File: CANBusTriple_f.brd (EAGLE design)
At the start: 50.2 x 49.5 mm, 63 parts, among them IC4 MCP1703CB, IC6 IC_MEM_23LC1024, U1 BLE112

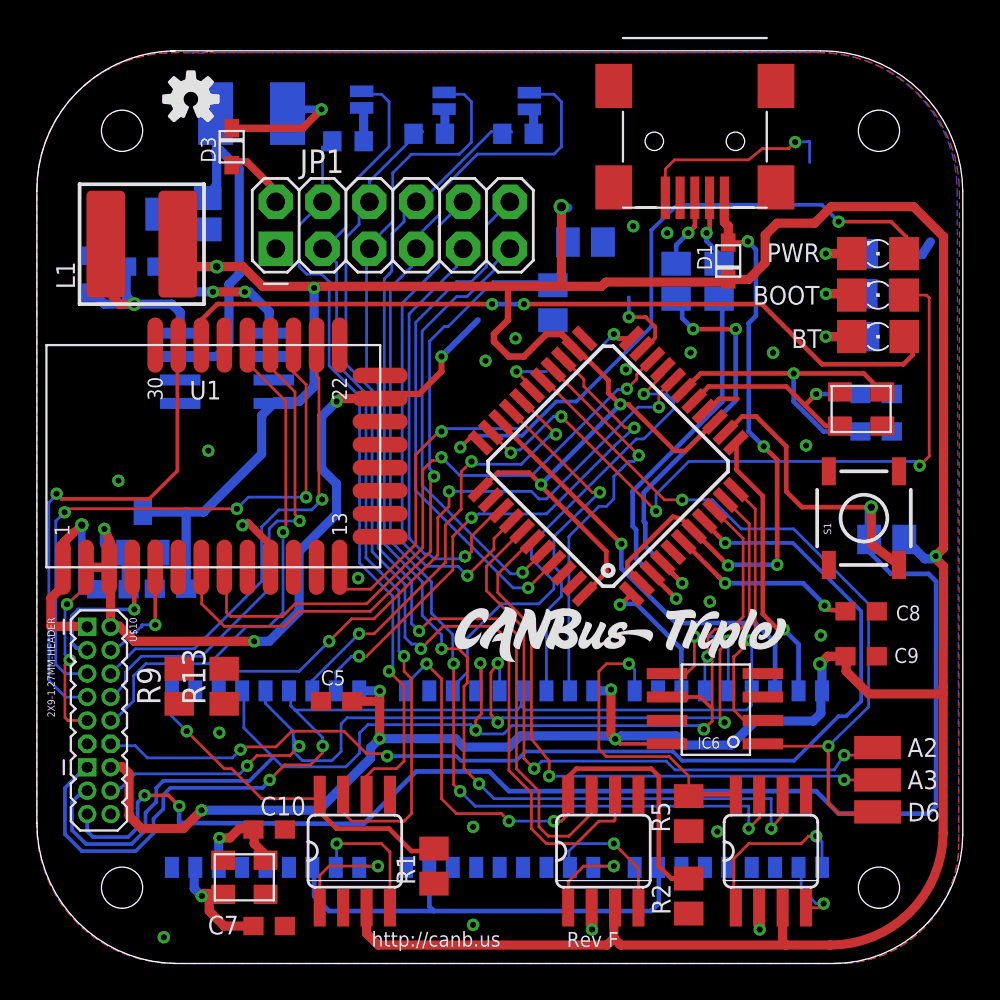
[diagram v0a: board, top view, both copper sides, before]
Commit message: Last sleep mode tweak, added line from BT LE to CAN1INT to wake the MCU up via BT
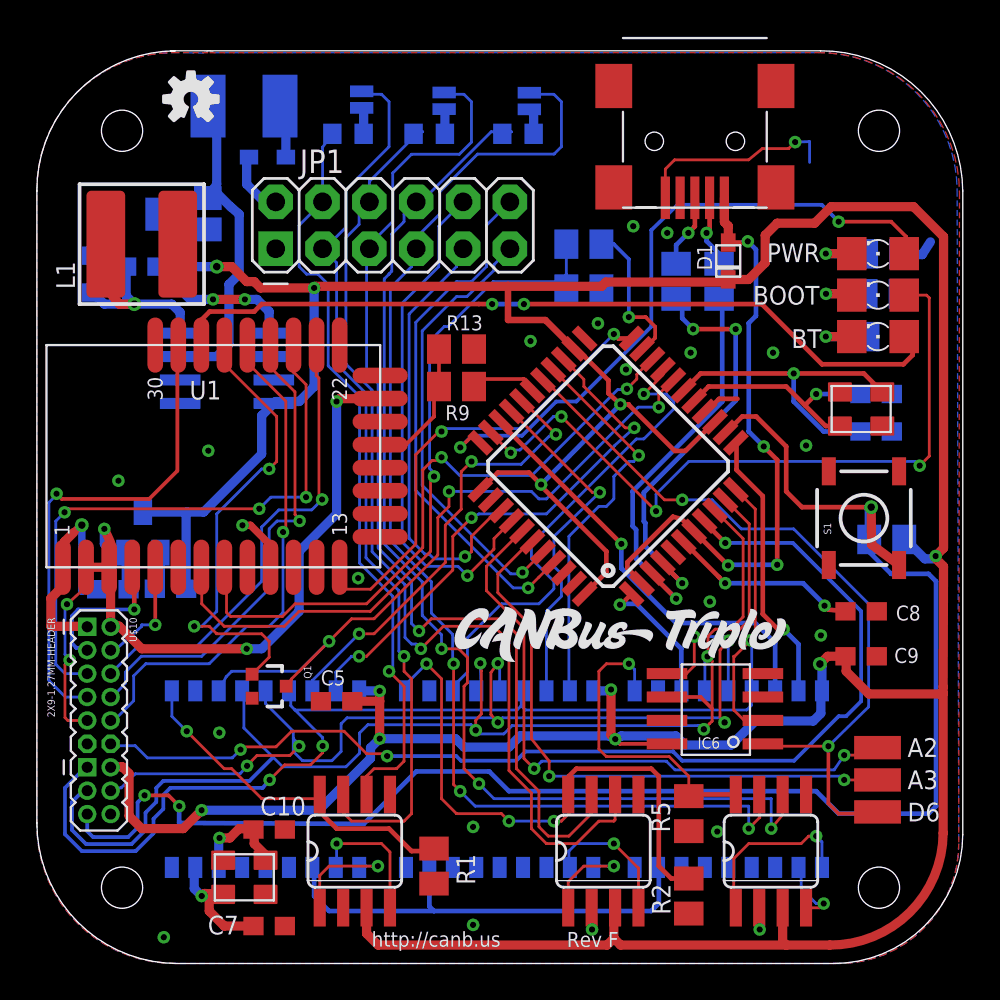
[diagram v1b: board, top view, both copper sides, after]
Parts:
- added Q1: MOSFET-NCHANNEL2N7002PW, SparkFun-DiscreteSemi:SOT323
- L1: value 47uH -> 68uH
- moved R13 22.2 mm to (22.8, 33.3), turned to 180 degrees
- moved R9 22.1 mm to (22.8, 31.3), turned to 0 degrees
- moved D3 2.02 mm to (12.5, 43.7), flipped to the bottom, turned to 180 degrees
- moved R10 1.83 mm to (29.7, 36.6), turned to 0 degrees
- moved F1 0.57 mm to (11.2, 46.5)
- moved CAN1-TRM 0.41 mm to (16.9, 45.0)
- moved R11 0.14 mm to (29.7, 39.0), turned to 180 degrees
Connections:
- new net N$33: Q1.1, U1.P0_1
- net +5V: no longer L1.2
- net CAN1_INT: now also Q1.3
- net GND: now also Q1.2
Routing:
- net N$33: track 0.00 -> 25.3 mm, vias 0 -> 2
- net +5V: track 259.0 -> 248.7 mm, vias 12 -> 11
- net +3V: track 58.8 -> 50.8 mm, vias 6 -> 5
- net N$29: track 0.00 -> 7.65 mm
- net N$22: track 7.25 -> 2.90 mm, vias 1 -> 0
- net N$19: track 4.28 -> 8.17 mm
- net CAN1_INT: track 34.2 -> 37.6 mm
- net N$38: track 36.0 -> 39.3 mm
- net GND: track 34.9 -> 36.9 mm
- net SUPPLY: track 19.1 -> 18.1 mm
- net N$36: track 3.21 -> 3.89 mm, vias 1 -> 0

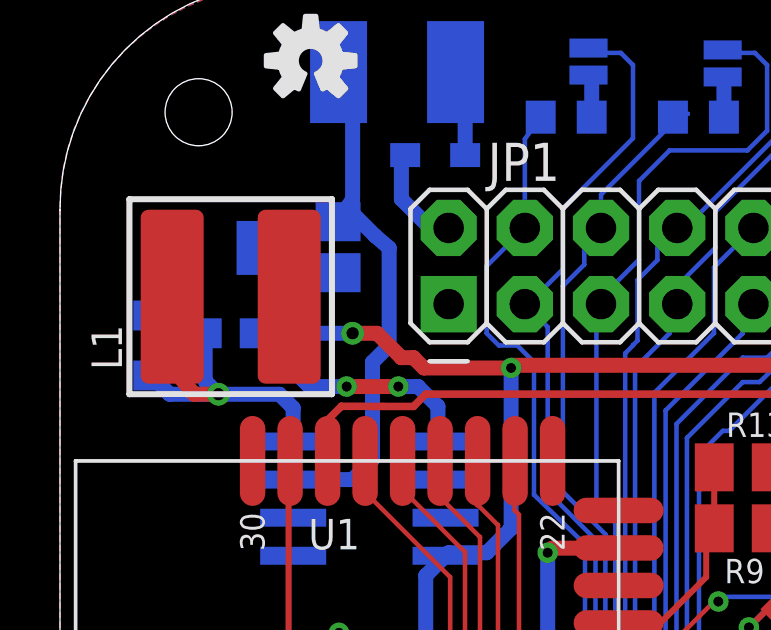
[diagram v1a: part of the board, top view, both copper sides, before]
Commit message: Fix missing trace on inductor
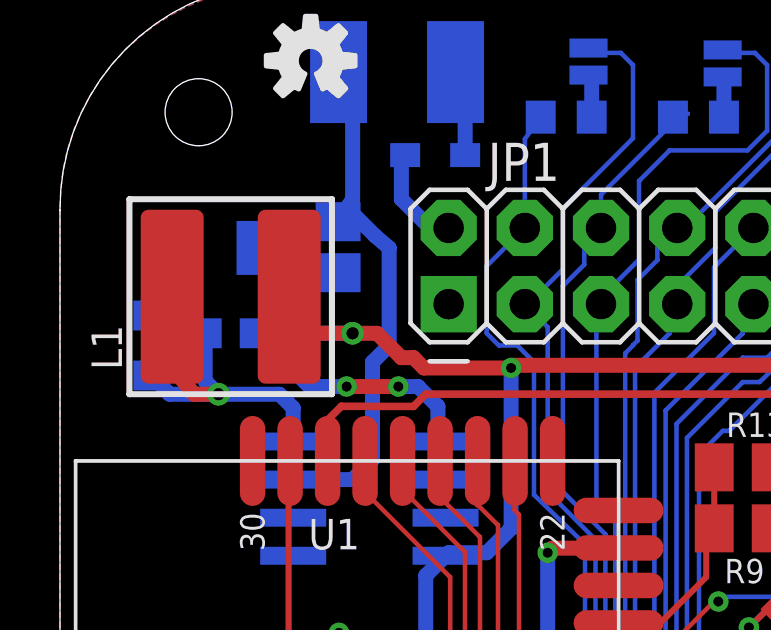
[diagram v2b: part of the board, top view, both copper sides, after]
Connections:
- net +5V: now also L1.2
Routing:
- net +5V: track 248.7 -> 251.5 mm
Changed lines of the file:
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@@
 <wire x1="11.3792" y1="36.9824" x2="10.5664" y2="37.7952" width="0.5" layer="1"/>
 <wire x1="10.5664" y1="37.7952" x2="9.7536" y2="37.7952" width="0.5" layer="1"/>
+<contactref element="L1" pad="2"/>
+<wire x1="7.6396" y1="39.0144" x2="7.6396" y2="38.69" width="0.5" layer="1"/>
+<wire x1="7.6396" y1="38.69" x2="8.5344" y2="37.7952" width="0.5" layer="1"/>
+<wire x1="8.5344" y1="37.7952" x2="9.7536" y2="37.7952" width="0.5" layer="1"/>
 </signal>
 <signal name="CAN1HIGH">
